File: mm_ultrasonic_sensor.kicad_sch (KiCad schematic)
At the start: 0 parts

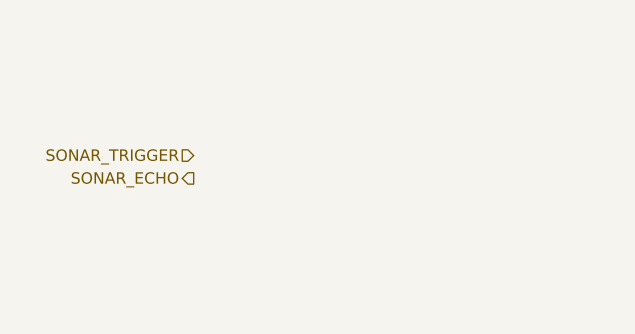
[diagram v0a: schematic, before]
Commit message: fin tp2
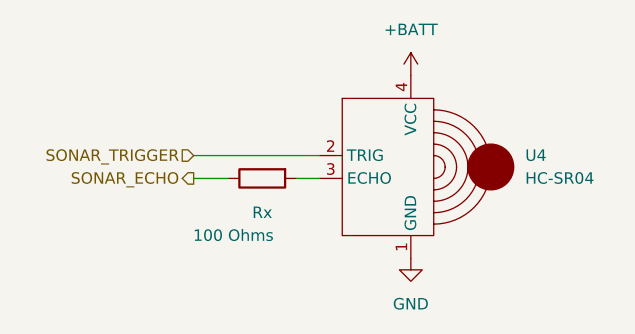
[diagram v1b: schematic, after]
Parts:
- added Rx: 100 Ohms, symbol Device:R
- added U4: HC-SR04, minimouse:HC-SR04, symbol minimouse:HC-SR04
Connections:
- net SONAR_ECHO: now also Rx.1
- net SONAR_TRIGGER: now also U4.2 (TRIG)
- new net: Rx.2, U4.3 (ECHO)
- new net +BATT: U4.4 (VCC)
- new net GND: U4.1 (GND)
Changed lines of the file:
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@@
 (kicad_sch (version 20230121) (generator eeschema)
   (paper "A4")
+  (wire (pts (xy 109.22 91.44) (xy 113.03 91.44))
+    (stroke (width 0) (type default))
+  )
+  (wire (pts (xy 109.22 88.9) (xy 123.19 88.9))
+    (stroke (width 0) (type default))
+  )
+  (wire (pts (xy 120.65 91.44) (xy 123.19 91.44))
+    (stroke (width 0) (type default))
+  )
   (hierarchical_label "SONAR_TRIGGER" (shape input) (at 109.22 88.9 180) (fields_autoplaced)
     (effects (font (size 1.27 1.27)) (justify right))
@@
     (effects (font (size 1.27 1.27)) (justify right))
   )
+  (symbol (lib_id "minimouse:HC-SR04") (at 133.35 90.17 0) (unit 1)
+    (in_bom yes) (on_board yes) (dnp no) (fields_autoplaced)
+    (property "Reference" "U4" (at 146.05 88.9 0)
+      (effects (font (size 1.27 1.27)) (justify left))
+    )
+    (property "Value" "HC-SR04" (at 146.05 91.44 0)
+      (effects (font (size 1.27 1.27)) (justify left))
+    )
+    (property "Footprint" "minimouse:HC-SR04" (at 133.35 90.17 0)
+      (effects (font (size 1.27 1.27)) hide)
+    )
+    (property "Datasheet" "" (at 133.35 90.17 0)
+      (effects (font (size 1.27 1.27)) hide)
+    )
+    (pin "4")
+    (pin "1")
+    (pin "2")
+    (pin "3")
+    (instances
+      (project "minimouse"
+        (path "/d8fa4cba-2469-4231-847f-065b6b829f44/224298a9-7d6e-4a70-a0a5-f2614895ec28"
+          (reference "U4") (unit 1)
+        )
+      )
+    )
+  )
+  (symbol (lib_id "power:+BATT") (at 133.35 80.01 0) (unit 1)
+    (in_bom yes) (on_board yes) (dnp no) (fields_autoplaced)
+    (property "Reference" "#PWR028" (at 133.35 83.82 0)
+      (effects (font (size 1.27 1.27)) hide)
+    )
+    (property "Value" "+BATT" (at 133.35 74.93 0)
+      (effects (font (size 1.27 1.27)))
+    )
+    (property "Footprint" "" (at 133.35 80.01 0)
+      (effects (font (size 1.27 1.27)) hide)
+    )
+    (property "Datasheet" "" (at 133.35 80.01 0)
+      (effects (font (size 1.27 1.27)) hide)
+    )
+    (pin "1")
+    (instances
+      (project "minimouse"
+        (path "/d8fa4cba-2469-4231-847f-065b6b829f44/224298a9-7d6e-4a70-a0a5-f2614895ec28"
+          (reference "#PWR028") (unit 1)
+        )
+      )
+    )
+  )
+  (symbol (lib_id "power:GND") (at 133.35 100.33 0) (unit 1)
+    (in_bom yes) (on_board yes) (dnp no) (fields_autoplaced)
+    (property "Reference" "#PWR029" (at 133.35 106.68 0)
+      (effects (font (size 1.27 1.27)) hide)
+    )
+    (property "Value" "GND" (at 133.35 105.41 0)
+      (effects (font (size 1.27 1.27)))
+    )
+    (property "Footprint" "" (at 133.35 100.33 0)
+      (effects (font (size 1.27 1.27)) hide)
+    )
+    (property "Datasheet" "" (at 133.35 100.33 0)
+      (effects (font (size 1.27 1.27)) hide)
+    )
+    (pin "1")
+    (instances
+      (project "minimouse"
+        (path "/d8fa4cba-2469-4231-847f-065b6b829f44/224298a9-7d6e-4a70-a0a5-f2614895ec28"
+          (reference "#PWR029") (unit 1)
+        )
+      )
+    )
+  )
+  (symbol (lib_id "Device:R") (at 116.84 91.44 90) (mirror x) (unit 1)
+    (in_bom yes) (on_board yes) (dnp no)
+    (property "Reference" "Rx" (at 116.84 95.25 90)
+      (effects (font (size 1.27 1.27)))
+    )
+    (property "Value" "100 Ohms" (at 118.11 97.79 90)
+      (effects (font (size 1.27 1.27)) (justify left))
+    )
+    (property "Footprint" "" (at 116.84 89.662 90)
+      (effects (font (size 1.27 1.27)) hide)
+    )
+    (property "Datasheet" "~" (at 116.84 91.44 0)
+      (effects (font (size 1.27 1.27)) hide)
+    )
+    (pin "2")
+    (pin "1")
+    (instances
+      (project "minimouse"
+        (path "/d8fa4cba-2469-4231-847f-065b6b829f44/d17bb1c7-f68a-465e-9a17-5858ef86fc30"
+          (reference "Rx") (unit 1)
+        )
+        (path "/d8fa4cba-2469-4231-847f-065b6b829f44/224298a9-7d6e-4a70-a0a5-f2614895ec28"
+          (reference "R10") (unit 1)
+        )
+      )
+    )
+  )
 )
